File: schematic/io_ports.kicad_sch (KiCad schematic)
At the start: 5 parts, among them J1 Cartridge Port, J2 Expansion Port

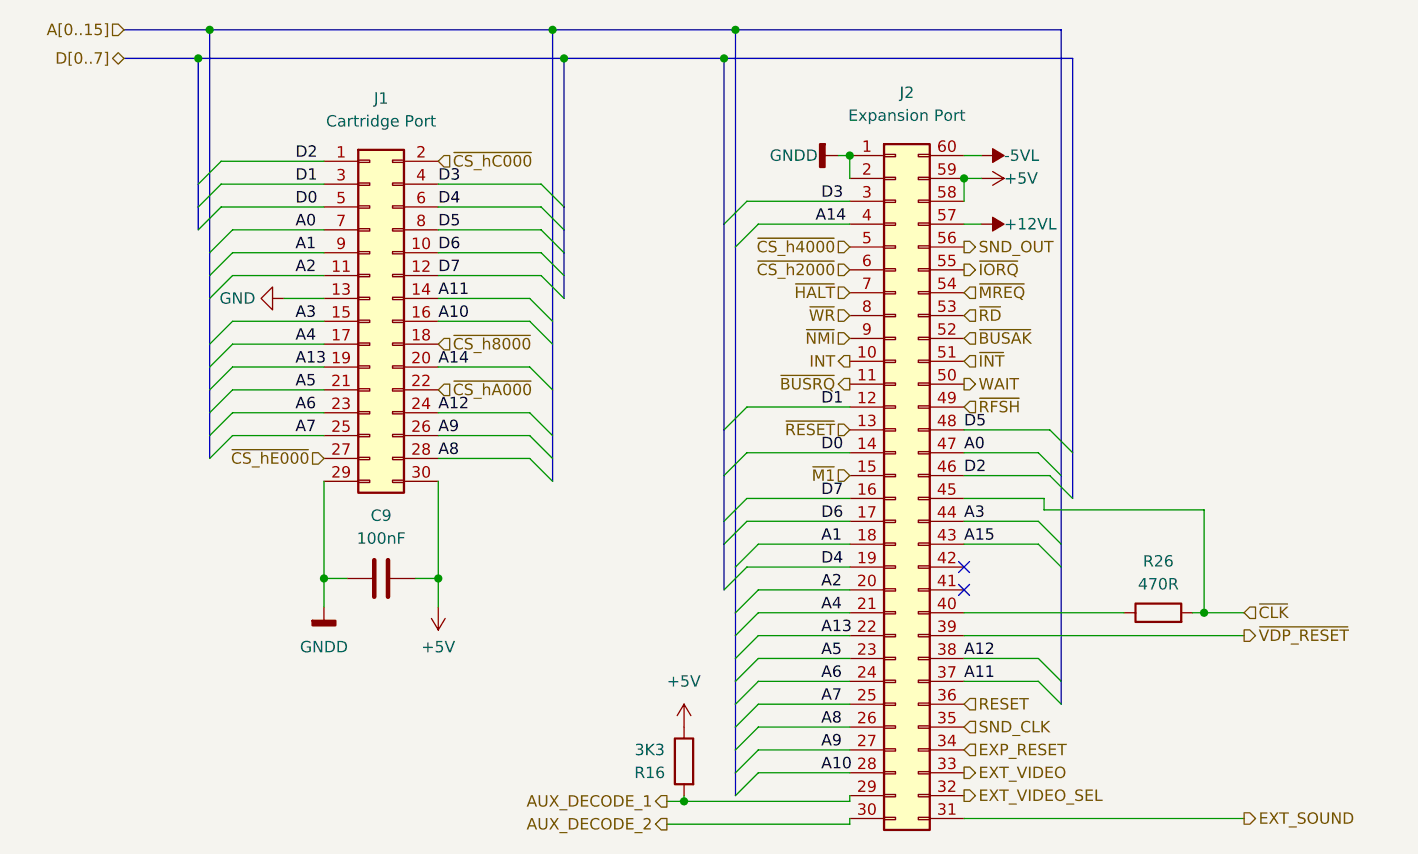
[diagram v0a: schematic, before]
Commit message: inital change to cpld
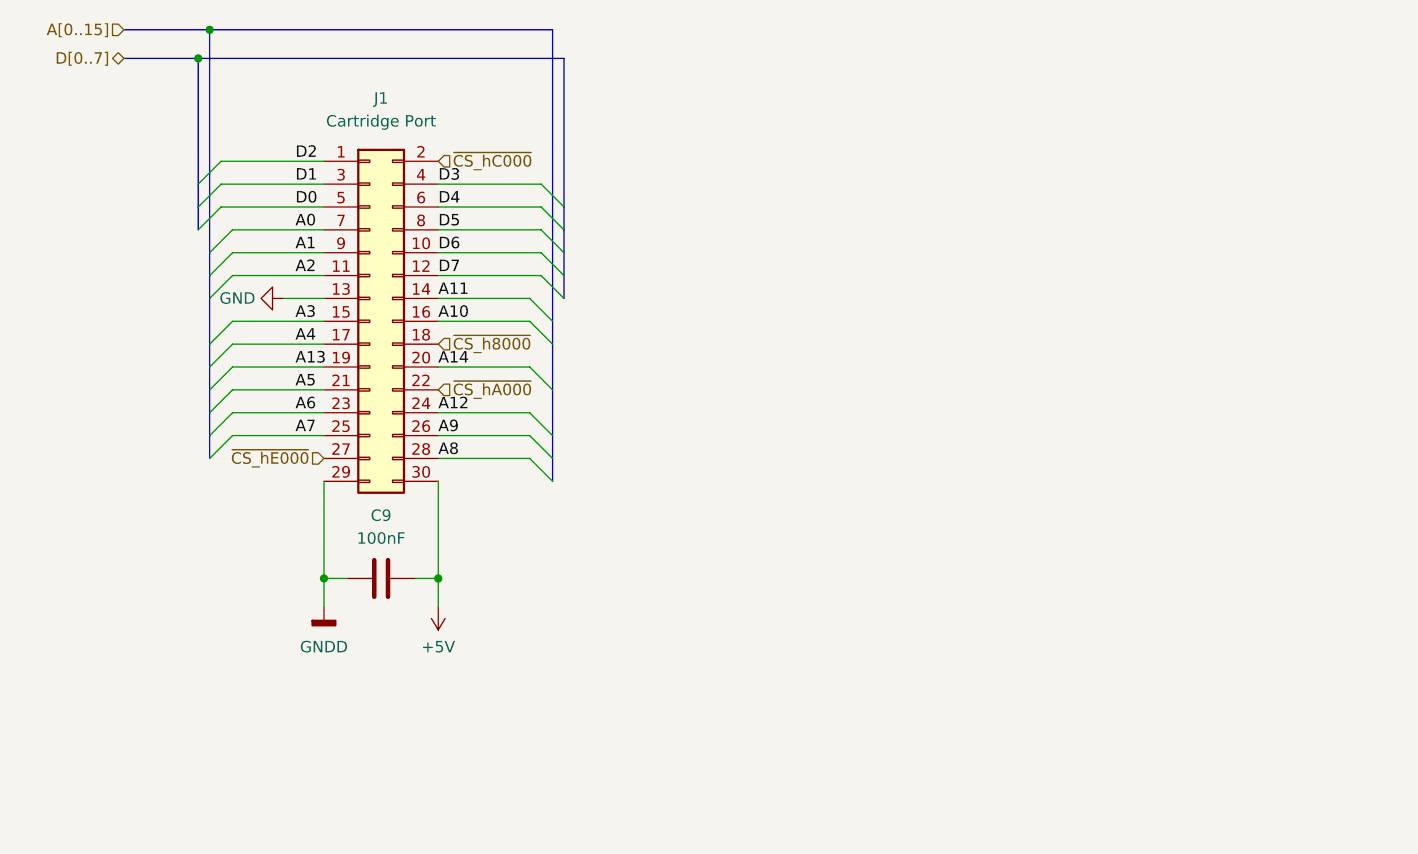
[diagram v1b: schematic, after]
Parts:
- removed J2: Expansion Port, Connector_PCBEdge_EXT:Colecovision_Expansion, symbol Connector_Generic:Conn_02x30_Counter_Clockwise
- removed R16: 3K3, Resistor_THT:R_Axial_DIN0207_L6.3mm_D2.5mm_P10.16mm_Horizontal, symbol Device:R
- removed R26: 470R, Resistor_THT:R_Axial_DIN0207_L6.3mm_D2.5mm_P10.16mm_Horizontal, symbol Device:R
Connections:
- no-connect marks 2 -> 0
